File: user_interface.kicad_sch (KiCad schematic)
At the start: 29 parts, among them CN5 Line out, CN6 Headphone, J2 SWD, J3 I2C, J6 SPI, J9 Serial, P1 GPIO, SW4 BTN1, SW5 BTN2

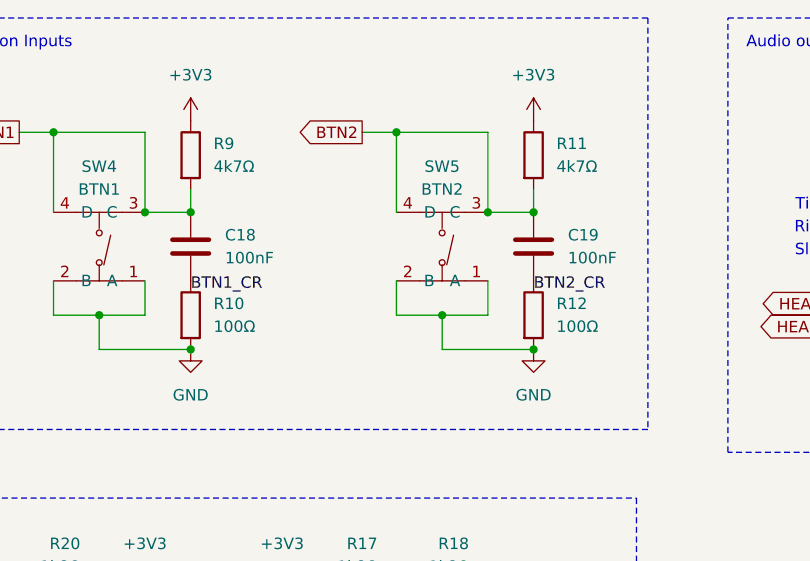
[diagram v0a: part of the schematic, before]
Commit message: Work on power section and some miscellaneous small areas
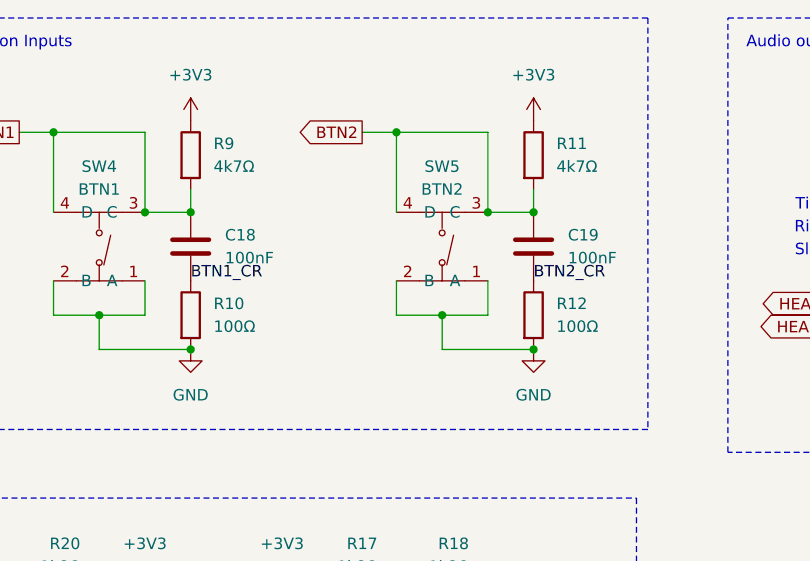
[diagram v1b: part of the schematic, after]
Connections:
- net BTN1_CR: now also C18.2, R10.1
- net BTN2_CR: now also C19.2, R12.1
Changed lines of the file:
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@@
 	)
 	(label "BTN1_CR"
-		(at 133.35 49.53 0)
+		(at 133.35 48.26 0)
 		(fields_autoplaced yes)
 		(effects
@@
 	)
 	(label "BTN2_CR"
-		(at 171.45 49.53 0)
+		(at 171.45 48.26 0)
 		(fields_autoplaced yes)
 		(effects
